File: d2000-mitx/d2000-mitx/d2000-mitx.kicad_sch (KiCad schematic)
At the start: 0 parts

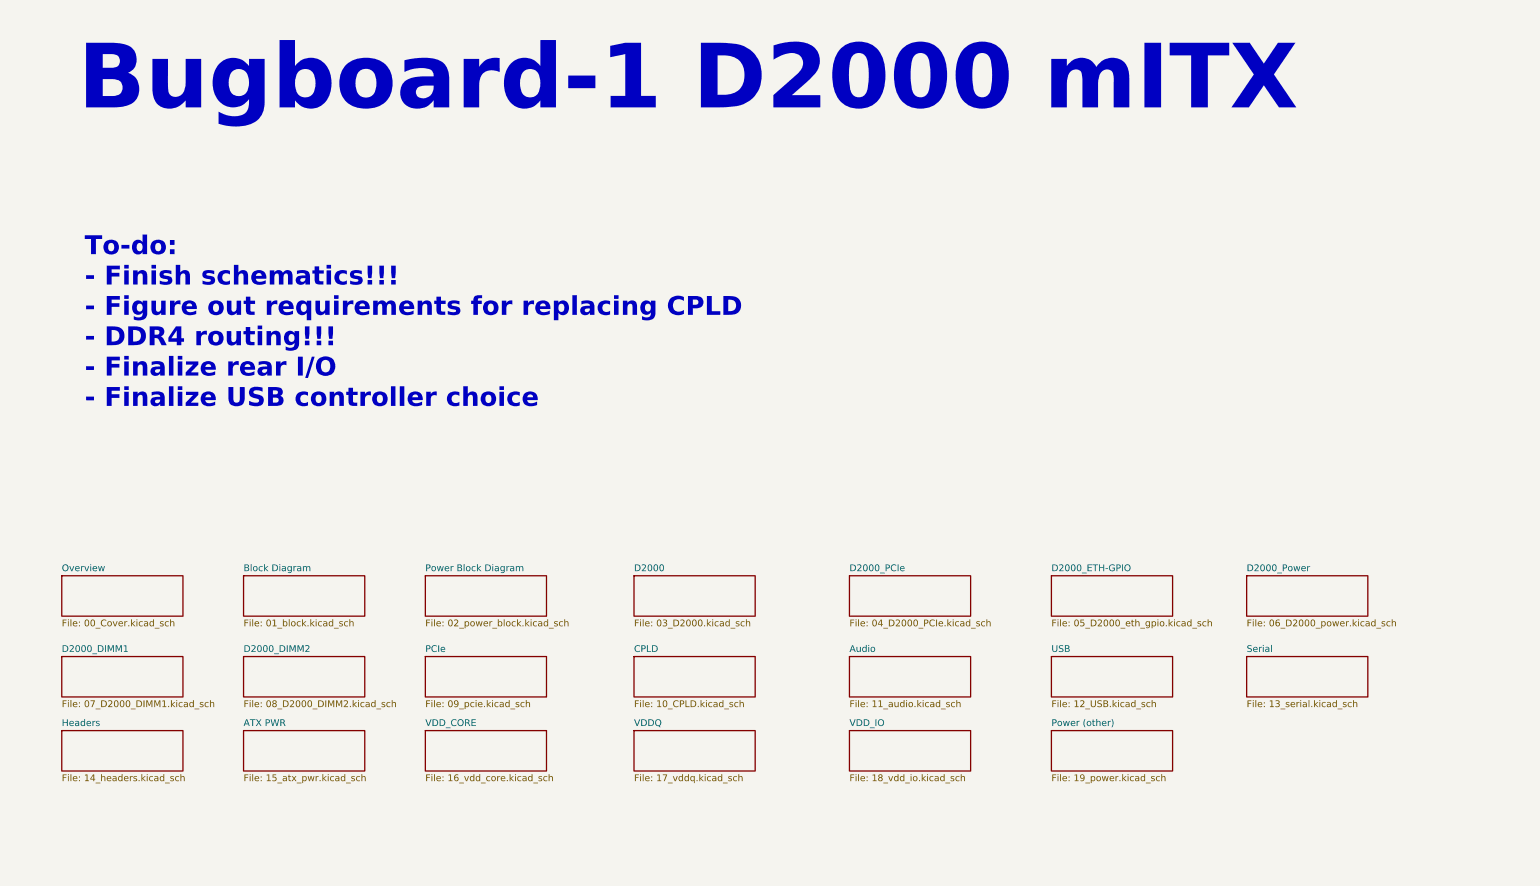
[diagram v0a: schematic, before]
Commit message: d2000-mitx
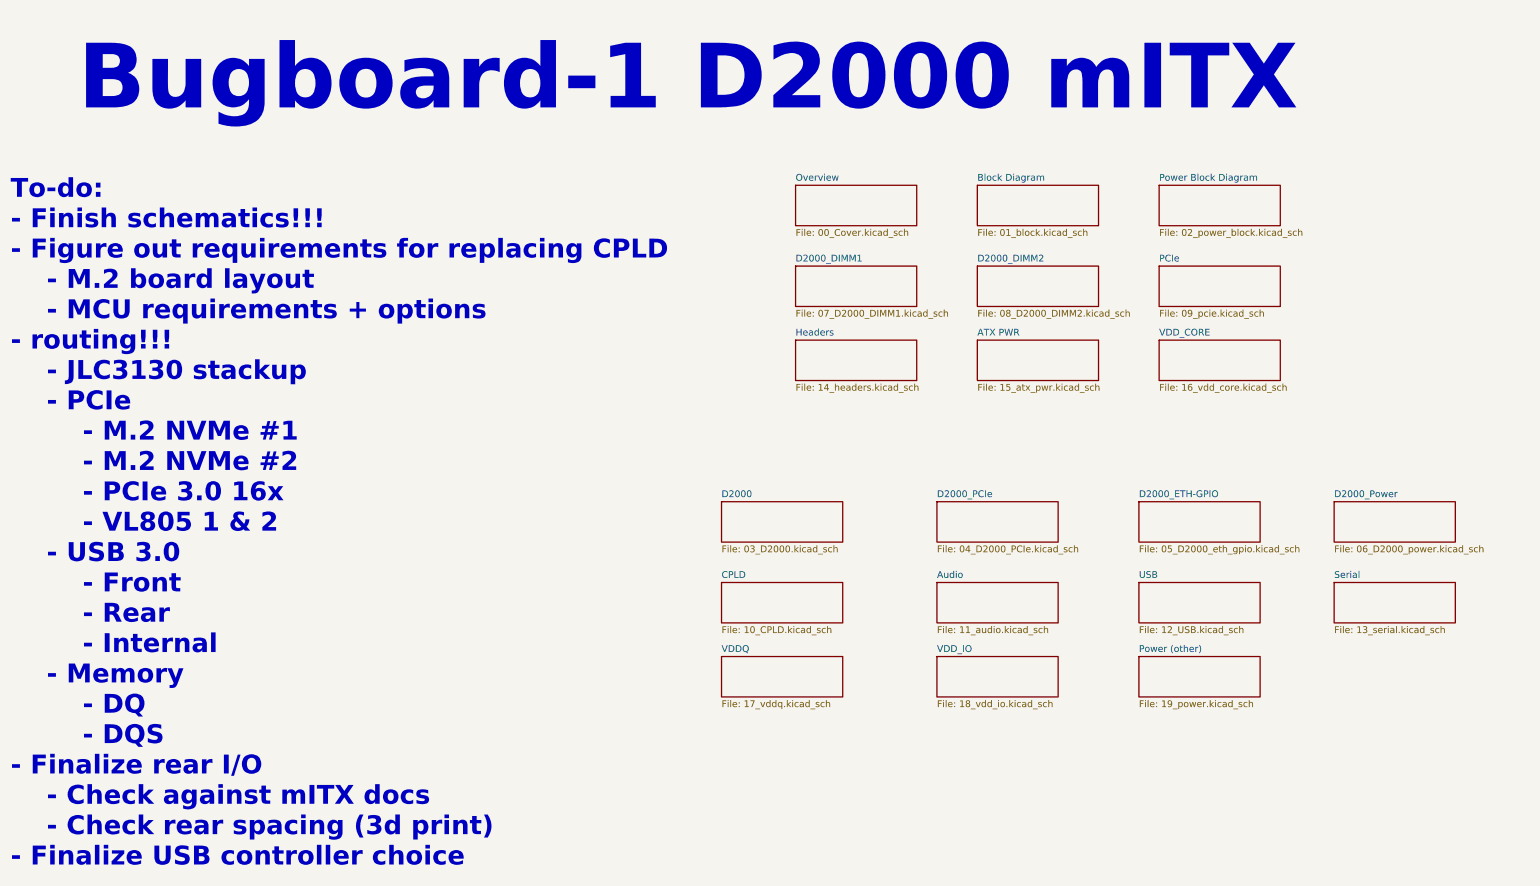
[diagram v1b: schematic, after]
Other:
- note added: "To-do: - Finish schematics!!! - Figure out requirements for replacing CPLD - M.2 board layout - MCU requirements + options - routing!!! - JLC3130 stackup - PCIe - M.2 NVMe #1 - M.2 NVMe #2 - PCIe 3.0 16x - VL805 1 & 2 - USB 3.0 - Front - Rear - Internal - Memory - DQ - DQS - Finalize rear I/O - Check against mITX docs - Check rear spacing (3d print) - Finalize USB controller choice"
- note removed: "To-do: - Finish schematics!!! - Figure out requirements for replacing CPLD - DDR4 routing!!! - Finalize rear I/O - Finalize USB controller choice"
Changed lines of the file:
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@@
 		)
 	)
-	(text "To-do:\n- Finish schematics!!!\n- Figure out requirements for replacing CPLD\n- DDR4 routing!!!\n- Finalize rear I/O\n- Finalize USB controller choice\n"
-		(exclude_from_sim no)
-		(at 30.988 75.438 0)
+	(text "To-do:\n- Finish schematics!!!\n- Figure out requirements for replacing CPLD\n	- M.2 board layout\n	- MCU requirements + options\n- routing!!!\n	- JLC3130 stackup\n	- PCIe\n		- M.2 NVMe #1\n		- M.2 NVMe #2\n		- PCIe 3.0 16x\n		- VL805 1 & 2\n	- USB 3.0\n		- Front\n		- Rear\n		- Internal\n	- Memory\n		- DQ\n		- DQS\n- Finalize rear I/O\n	- Check against mITX docs\n	- Check rear spacing (3d print)\n- Finalize USB controller choice\n"
+		(exclude_from_sim no)
+		(at 17.018 113.284 0)
 		(effects
 			(font
@@
 	)
 	(sheet
-		(at 26.67 138.43)
+		(at 165.1 64.77)
 		(size 22.86 7.62)
 		(exclude_from_sim no)
@@
 		)
 		(property "Sheetname" "D2000_DIMM1"
-			(at 26.67 137.7184 0)
+			(at 165.1 64.0584 0)
 			(effects
 				(font
@@
 		)
 		(property "Sheetfile" "07_D2000_DIMM1.kicad_sch"
-			(at 26.67 146.6346 0)
+			(at 165.1 72.9746 0)
 			(effects
 				(font
@@
 	)
 	(sheet
-		(at 250.19 123.19)
+		(at 266.7 109.22)
 		(size 22.86 7.62)
 		(exclude_from_sim no)
@@
 		)
 		(property "Sheetname" "D2000_Power"
-			(at 250.19 122.4784 0)
+			(at 266.7 108.5084 0)
 			(effects
 				(font
@@
 		)
 		(property "Sheetfile" "06_D2000_power.kicad_sch"
-			(at 250.19 131.3946 0)
+			(at 266.7 117.4246 0)
 			(effects
 				(font
@@
 	)
 	(sheet
-		(at 213.36 123.19)
+		(at 229.87 109.22)
 		(size 22.86 7.62)
 		(exclude_from_sim no)
@@
 		)
 		(property "Sheetname" "D2000_ETH-GPIO"
-			(at 213.36 122.4784 0)
+			(at 229.87 108.5084 0)
 			(effects
 				(font
@@
 		)
 		(property "Sheetfile" "05_D2000_eth_gpio.kicad_sch"
-			(at 213.36 131.3946 0)
+			(at 229.87 117.4246 0)
 			(effects
 				(font
@@
 	)
 	(sheet
-		(at 134.62 123.19)
+		(at 151.13 109.22)
 		(size 22.86 7.62)
 		(exclude_from_sim no)
@@
 		)
 		(property "Sheetname" "D2000"
-			(at 134.62 122.4784 0)
+			(at 151.13 108.5084 0)
 			(effects
 				(font
@@
 		)
 		(property "Sheetfile" "03_D2000.kicad_sch"
-			(at 134.62 131.3946 0)
+			(at 151.13 117.4246 0)
 			(effects
 				(font
@@
 	)
 	(sheet
-		(at 134.62 138.43)
+		(at 151.13 124.46)
 		(size 22.86 7.62)
 		(exclude_from_sim no)
@@
 		)
 		(property "Sheetname" "CPLD"
-			(at 134.62 137.7184 0)
+			(at 151.13 123.7484 0)
 			(effects
 				(font
@@
 		)
 		(property "Sheetfile" "10_CPLD.kicad_sch"
-			(at 134.62 146.6346 0)
+			(at 151.13 132.6646 0)
 			(effects
 				(font
@@
 	)
 	(sheet
-		(at 175.26 123.19)
+		(at 191.77 109.22)
 		(size 22.86 7.62)
 		(exclude_from_sim no)
@@
 		)
 		(property "Sheetname" "D2000_PCIe"
-			(at 175.26 122.4784 0)
+			(at 191.77 108.5084 0)
 			(effects
 				(font
@@
 		)
 		(property "Sheetfile" "04_D2000_PCIe.kicad_sch"
-			(at 175.26 131.3946 0)
+			(at 191.77 117.4246 0)
 			(effects
 				(font
@@
 	)
 	(sheet
-		(at 134.62 152.4)
+		(at 151.13 138.43)
 		(size 22.86 7.62)
 		(exclude_from_sim no)
@@
 		)
 		(property "Sheetname" "VDDQ"
-			(at 134.62 151.6884 0)
+			(at 151.13 137.7184 0)
 			(effects
 				(font
@@
 		)
 		(property "Sheetfile" "17_vddq.kicad_sch"
-			(at 134.62 160.6046 0)
+			(at 151.13 146.6346 0)
 			(effects
 				(font
@@
 	)
 	(sheet
-		(at 175.26 152.4)
+		(at 191.77 138.43)
 		(size 22.86 7.62)
 		(exclude_from_sim no)
@@
 		)
 		(property "Sheetname" "VDD_IO"
-			(at 175.26 151.6884 0)
+			(at 191.77 137.7184 0)
 			(effects
 				(font
@@
 		)
 		(property "Sheetfile" "18_vdd_io.kicad_sch"
-			(at 175.26 160.6046 0)
+			(at 191.77 146.6346 0)
 			(effects
 				(font
@@
 	)
 	(sheet
-		(at 213.36 152.4)
+		(at 229.87 138.43)
 		(size 22.86 7.62)
 		(exclude_from_sim no)
@@
 		)
 		(property "Sheetname" "Power (other)"
-			(at 213.36 151.6884 0)
+			(at 229.87 137.7184 0)
 			(effects
 				(font
@@
 		)
 		(property "Sheetfile" "19_power.kicad_sch"
-			(at 213.36 160.6046 0)
+			(at 229.87 146.6346 0)
 			(effects
 				(font
@@
 	)
 	(sheet
-		(at 95.25 152.4)
+		(at 233.68 78.74)
 		(size 22.86 7.62)
 		(exclude_from_sim no)
@@
 		)
 		(property "Sheetname" "VDD_CORE"
-			(at 95.25 151.6884 0)
+			(at 233.68 78.0284 0)
 			(effects
 				(font
@@
 		)
 		(property "Sheetfile" "16_vdd_core.kicad_sch"
-			(at 95.25 160.6046 0)
+			(at 233.68 86.9446 0)
 			(effects
 				(font
@@
 	)
 	(sheet
-		(at 213.36 138.43)
+		(at 229.87 124.46)
 		(size 22.86 7.62)
 		(exclude_from_sim no)
@@
 		)
 		(property "Sheetname" "USB"
-			(at 213.36 137.7184 0)
+			(at 229.87 123.7484 0)
 			(effects
 				(font
@@
 		)
 		(property "Sheetfile" "12_USB.kicad_sch"
-			(at 213.36 146.6346 0)
+			(at 229.87 132.6646 0)
 			(effects
 				(font
@@
 	)
 	(sheet
-		(at 26.67 123.19)
+		(at 165.1 49.53)
 		(size 22.86 7.62)
 		(exclude_from_sim no)
@@
 		)
 		(property "Sheetname" "Overview"
-			(at 26.67 122.4784 0)
+			(at 165.1 48.8184 0)
 			(effects
 				(font
@@
 		)
 		(property "Sheetfile" "00_Cover.kicad_sch"
-			(at 26.67 131.3946 0)
+			(at 165.1 57.7346 0)
 			(effects
 				(font
@@
 	)
 	(sheet
-		(at 250.19 138.43)
+		(at 266.7 124.46)
 		(size 22.86 7.62)
 		(exclude_from_sim no)
@@
 		)
 		(property "Sheetname" "Serial"
-			(at 250.19 137.7184 0)
+			(at 266.7 123.7484 0)
 			(effects
 				(font
@@
 		)
 		(property "Sheetfile" "13_serial.kicad_sch"
-			(at 250.19 146.6346 0)
+			(at 266.7 132.6646 0)
 			(effects
 				(font
@@
 	)
 	(sheet
-		(at 175.26 138.43)
+		(at 191.77 124.46)
 		(size 22.86 7.62)
 		(exclude_from_sim no)
@@
 		)
 		(property "Sheetname" "Audio"
-			(at 175.26 137.7184 0)
+			(at 191.77 123.7484 0)
 			(effects
 				(font
@@
 		)
 		(property "Sheetfile" "11_audio.kicad_sch"
-			(at 175.26 146.6346 0)
+			(at 191.77 132.6646 0)
 			(effects
 				(font
@@
 	)
 	(sheet
-		(at 60.96 152.4)
+		(at 199.39 78.74)
 		(size 22.86 7.62)
 		(exclude_from_sim no)
@@
 		)
 		(property "Sheetname" "ATX PWR"
-			(at 60.96 151.6884 0)
+			(at 199.39 78.0284 0)
 			(effects
 				(font
@@
 		)
 		(property "Sheetfile" "15_atx_pwr.kicad_sch"
-			(at 60.96 160.6046 0)
+			(at 199.39 86.9446 0)
 			(effects
 				(font
@@
 	)
 	(sheet
-		(at 60.96 138.43)
+		(at 199.39 64.77)
 		(size 22.86 7.62)
 		(exclude_from_sim no)
@@
 		)
 		(property "Sheetname" "D2000_DIMM2"
-			(at 60.96 137.7184 0)
+			(at 199.39 64.0584 0)
 			(effects
 				(font
@@
 		)
 		(property "Sheetfile" "08_D2000_DIMM2.kicad_sch"
-			(at 60.96 146.6346 0)
+			(at 199.39 72.9746 0)
 			(effects
 				(font
@@
 	)
 	(sheet
-		(at 60.96 123.19)
+		(at 199.39 49.53)
 		(size 22.86 7.62)
 		(exclude_from_sim no)
@@
 		)
 		(property "Sheetname" "Block Diagram"
-			(at 60.96 122.4784 0)
+			(at 199.39 48.8184 0)
 			(effects
 				(font
@@
 		)
 		(property "Sheetfile" "01_block.kicad_sch"
-			(at 60.96 131.3946 0)
+			(at 199.39 57.7346 0)
 			(effects
 				(font
@@
 	)
 	(sheet
-		(at 95.25 138.43)
+		(at 233.68 64.77)
 		(size 22.86 7.62)
 		(exclude_from_sim no)
@@
 		)
 		(property "Sheetname" "PCIe"
-			(at 95.25 137.7184 0)
+			(at 233.68 64.0584 0)
 			(effects
 				(font
@@
 		)
 		(property "Sheetfile" "09_pcie.kicad_sch"
-			(at 95.25 146.6346 0)
+			(at 233.68 72.9746 0)
 			(effects
 				(font
@@
 	)
 	(sheet
-		(at 95.25 123.19)
+		(at 233.68 49.53)
 		(size 22.86 7.62)
 		(exclude_from_sim no)
@@
 		)
 		(property "Sheetname" "Power Block Diagram"
-			(at 95.25 122.4784 0)
+			(at 233.68 48.8184 0)
 			(effects
 				(font
@@
 		)
 		(property "Sheetfile" "02_power_block.kicad_sch"
-			(at 95.25 131.3946 0)
+			(at 233.68 57.7346 0)
 			(effects
 				(font
@@
 	)
 	(sheet
-		(at 26.67 152.4)
+		(at 165.1 78.74)
 		(size 22.86 7.62)
 		(exclude_from_sim no)
@@
 		)
 		(property "Sheetname" "Headers"
-			(at 26.67 151.6884 0)
+			(at 165.1 78.0284 0)
 			(effects
 				(font
@@
 		)
 		(property "Sheetfile" "14_headers.kicad_sch"
-			(at 26.67 160.6046 0)
-			(effects
-				(font
+			(at 165.1 86.9446 0)
+			(effects
+				(font
